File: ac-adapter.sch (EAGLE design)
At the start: 88 parts, among them IC1 UCC256404A, IC2 TL431, Q1 300V 5A, Q2 300V 5A, Q3 TLP621-1, T1 COMMON_FILTER-SU10VFC, T2 TRANSFORMAER_FLYBACK-ETD34

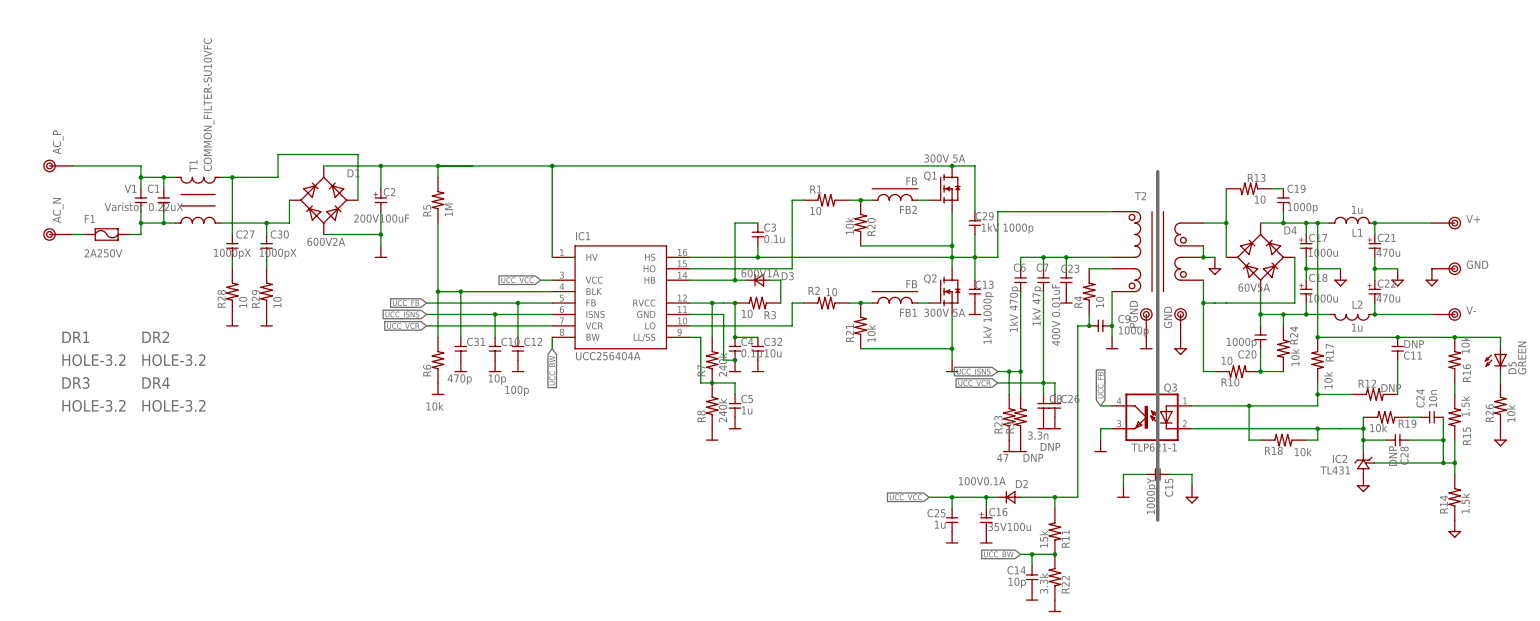
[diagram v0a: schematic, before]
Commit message: GaN
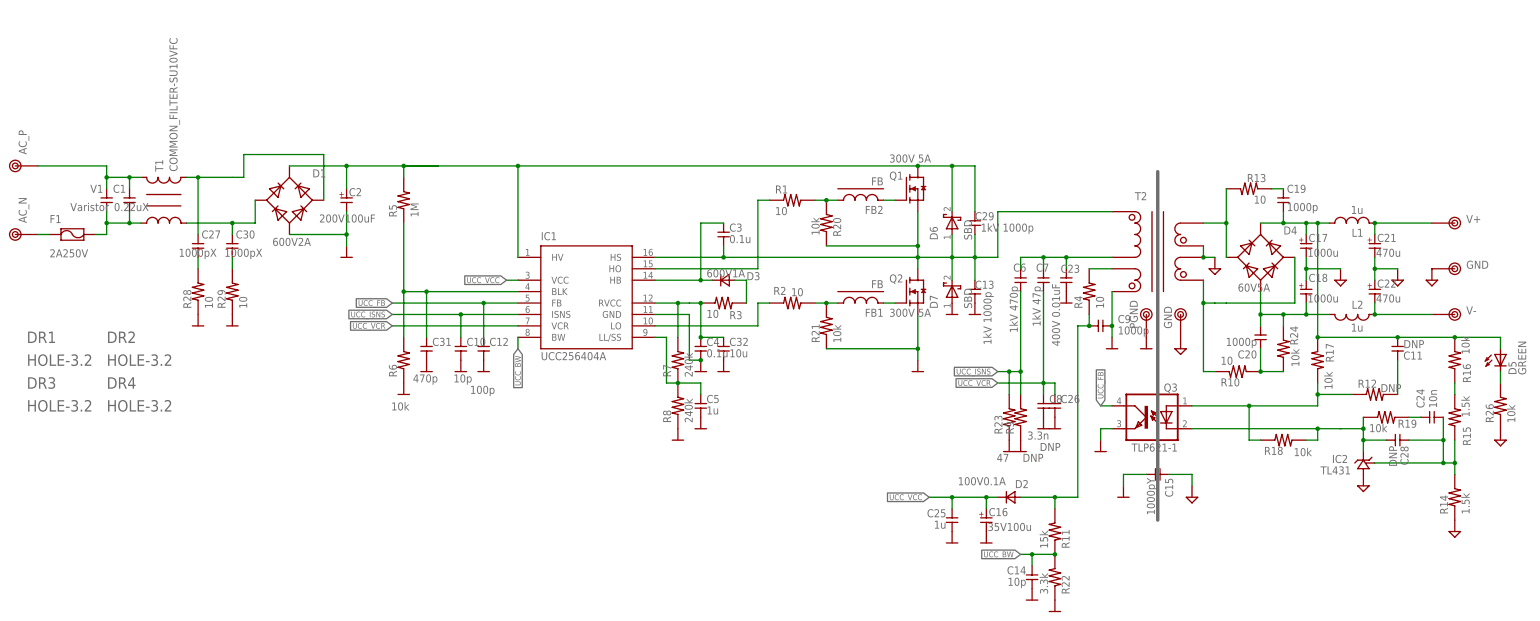
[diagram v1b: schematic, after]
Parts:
- added D6, D7: SBD, my_rcl:SBD-1A2
- Q1, Q2: device my_ic:NMOS-DFN -> my_ic:NMOS-GAN
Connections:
- net PGND: now also D7.A
- net SW: now also D6.A, D7.K
- net VH: now also D6.K
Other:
- moved on the sheet: C1, C10, C12, C2, C27, C3, C30, C31, C32, C4, C5, D1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
